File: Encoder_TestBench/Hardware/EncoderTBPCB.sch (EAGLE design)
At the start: 18 parts, among them IC1 7805DT, U1 ATMEGA328P-PU

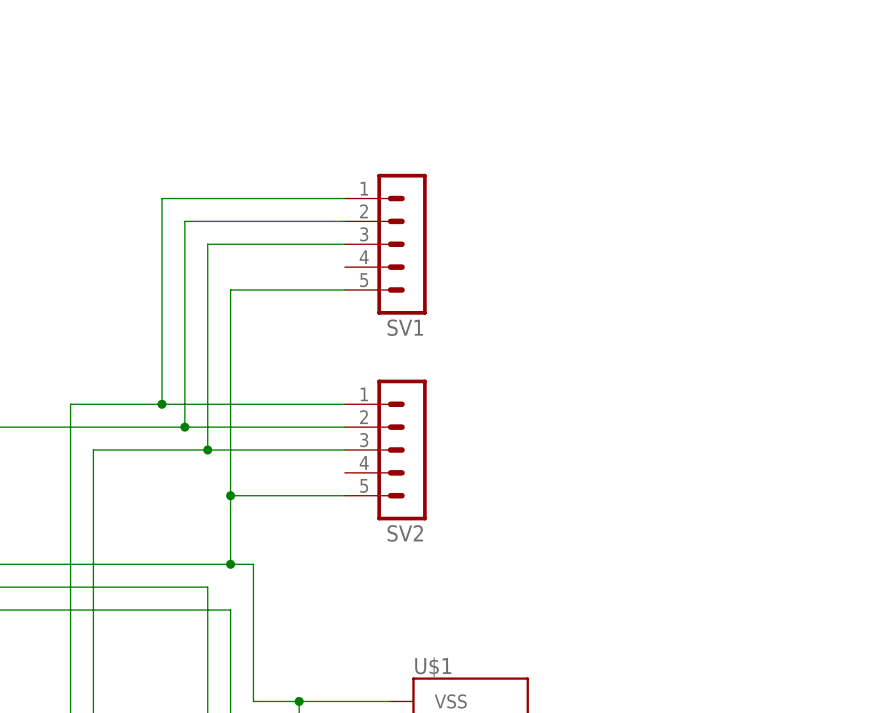
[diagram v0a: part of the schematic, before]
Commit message: Board Revised
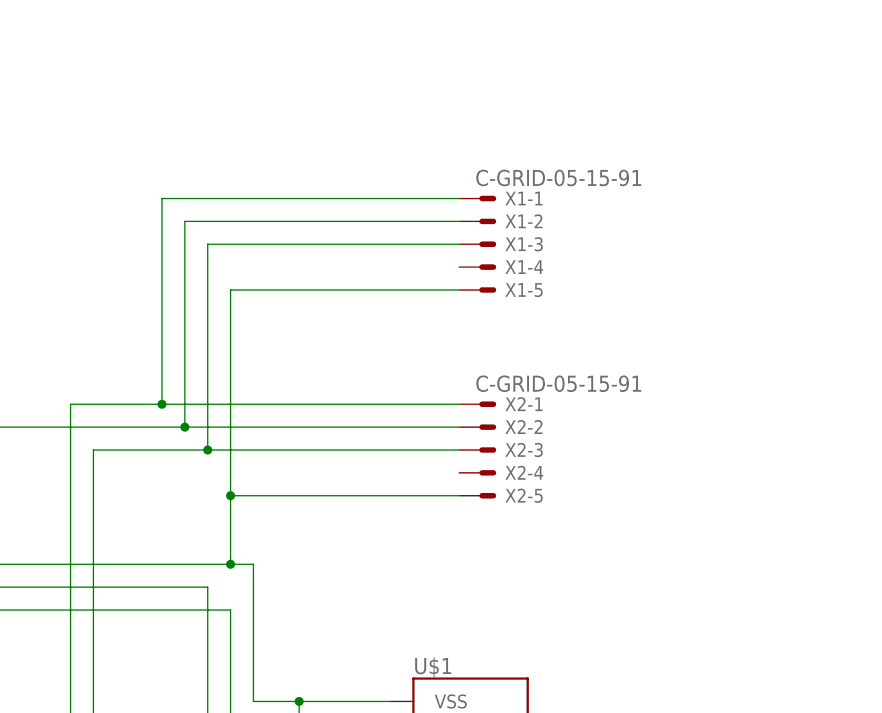
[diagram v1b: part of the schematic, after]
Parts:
- removed SV1, SV2: (no value), con-lstb:MA05-1
- added X1, X2: C-GRID-05-15-91, con-molex:C-GRID-05-15-91
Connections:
- net N$13: now also X1-1.S, X2-1.S; no longer SV1.1, SV2.1
- net N$14: now also X1-3.S, X2-3.S; no longer SV1.3, SV2.3
- net VDD: now also X1-2.S, X2-2.S; no longer SV1.2, SV2.2
- net VSS: now also X1-5.S, X2-5.S; no longer SV1.5, SV2.5
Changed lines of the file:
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@@
 <part name="R3" library="resistor" deviceset="R-US_" device="R0603" value="1MΩ"/>
 <part name="R4" library="resistor" deviceset="R-US_" device="R0603" value="850Ω"/>
-<part name="SV1" library="con-lstb" deviceset="MA05-1" device=""/>
-<part name="SV2" library="con-lstb" deviceset="MA05-1" device=""/>
 <part name="U$1" library="HD44780LCD" deviceset="LCD-HD44780" device="16X2-4-HOLES" technology="4-HOLES"/>
 <part name="R2" library="resistor" deviceset="R-US_" device="R0603" value="200Ω"/>
+<part name="X1" library="con-molex" deviceset="C-GRID-05" device="-15-91"/>
+<part name="X2" library="con-molex" deviceset="C-GRID-05" device="-15-91"/>
 </parts>
 <sheets>
@@
 <instance part="R3" gate="G$1" x="-5.08" y="43.18" rot="R90"/>
 <instance part="R4" gate="G$1" x="78.74" y="22.86" rot="R90"/>
-<instance part="SV1" gate="G$1" x="101.6" y="124.46" rot="R180"/>
-<instance part="SV2" gate="G$1" x="101.6" y="101.6" rot="R180"/>
 <instance part="U$1" gate="G$1" x="109.22" y="53.34"/>
 <instance part="R2" gate="G$1" x="66.04" y="15.24" rot="R180"/>
+<instance part="X1" gate="-1" x="109.22" y="129.54"/>
+<instance part="X1" gate="-2" x="109.22" y="127"/>
+<instance part="X1" gate="-3" x="109.22" y="124.46"/>
+<instance part="X1" gate="-4" x="109.22" y="121.92"/>
+<instance part="X1" gate="-5" x="109.22" y="119.38"/>
+<instance part="X2" gate="-1" x="109.22" y="106.68"/>
+<instance part="X2" gate="-2" x="109.22" y="104.14"/>
+<instance part="X2" gate="-3" x="109.22" y="101.6"/>
+<instance part="X2" gate="-4" x="109.22" y="99.06"/>
+<instance part="X2" gate="-5" x="109.22" y="96.52"/>
 </instances>
 <busses>
@@
 <junction x="81.28" y="88.9"/>
 <wire x1="81.28" y1="96.52" x2="81.28" y2="119.38" width="0.1524" layer="91"/>
-<wire x1="81.28" y1="96.52" x2="93.98" y2="96.52" width="0.1524" layer="91"/>
 <junction x="81.28" y="96.52"/>
 <wire x1="96.52" y1="5.08" x2="96.52" y2="35.56" width="0.1524" layer="91"/>
 <wire x1="96.52" y1="35.56" x2="99.06" y2="35.56" width="0.1524" layer="91"/>
-<pinref part="SV2" gate="G$1" pin="5"/>
 <pinref part="U1" gate="A" pin="GND_2"/>
 <pinref part="U1" gate="A" pin="GND"/>
@@
 <pinref part="U$1" gate="G$1" pin="R/W"/>
 <pinref part="U$1" gate="G$1" pin="VSS"/>
-<pinref part="SV1" gate="G$1" pin="5"/>
-<wire x1="81.28" y1="119.38" x2="93.98" y2="119.38" width="0.1524" layer="91"/>
 <pinref part="R2" gate="G$1" pin="2"/>
 <wire x1="60.96" y1="15.24" x2="58.42" y2="15.24" width="0.1524" layer="91"/>
 <junction x="58.42" y="15.24"/>
+<pinref part="X1" gate="-5" pin="S"/>
+<wire x1="81.28" y1="119.38" x2="106.68" y2="119.38" width="0.1524" layer="91"/>
+<pinref part="X2" gate="-5" pin="S"/>
+<wire x1="81.28" y1="96.52" x2="106.68" y2="96.52" width="0.1524" layer="91"/>
 </segment>
 <segment>
@@
 <wire x1="17.78" y1="104.14" x2="76.2" y2="104.14" width="0.1524" layer="91"/>
 <pinref part="JP1" gate="A" pin="2"/>
-<wire x1="76.2" y1="104.14" x2="93.98" y2="104.14" width="0.1524" layer="91"/>
+<wire x1="76.2" y1="104.14" x2="106.68" y2="104.14" width="0.1524" layer="91"/>
 <wire x1="2.54" y1="22.86" x2="7.62" y2="22.86" width="0.1524" layer="91"/>
 <wire x1="7.62" y1="22.86" x2="7.62" y2="27.94" width="0.1524" layer="91"/>
@@
 <wire x1="76.2" y1="104.14" x2="76.2" y2="127" width="0.1524" layer="91"/>
 <junction x="76.2" y="104.14"/>
-<wire x1="76.2" y1="127" x2="93.98" y2="127" width="0.1524" layer="91"/>
+<wire x1="76.2" y1="127" x2="106.68" y2="127" width="0.1524" layer="91"/>
 <pinref part="P+2" gate="1" pin="+5V"/>
-<pinref part="SV1" gate="G$1" pin="2"/>
-<pinref part="SV2" gate="G$1" pin="2"/>
 <wire x1="17.78" y1="73.66" x2="19.05" y2="73.66" width="0.1524" layer="91"/>
 <pinref part="U1" gate="A" pin="VCC"/>
 <pinref part="U1" gate="A" pin="AVCC"/>
+<pinref part="X1" gate="-2" pin="S"/>
+<pinref part="X2" gate="-2" pin="S"/>
 </segment>
 </net>
@@
 <segment>
 <wire x1="63.5" y1="106.68" x2="73.66" y2="106.68" width="0.1524" layer="91"/>
-<wire x1="73.66" y1="106.68" x2="93.98" y2="106.68" width="0.1524" layer="91"/>
+<wire x1="73.66" y1="106.68" x2="106.68" y2="106.68" width="0.1524" layer="91"/>
 <wire x1="73.66" y1="106.68" x2="73.66" y2="129.54" width="0.1524" layer="91"/>
 <junction x="73.66" y="106.68"/>
-<wire x1="73.66" y1="129.54" x2="93.98" y2="129.54" width="0.1524" layer="91"/>
-<pinref part="SV1" gate="G$1" pin="1"/>
-<pinref part="SV2" gate="G$1" pin="1"/>
+<wire x1="73.66" y1="129.54" x2="106.68" y2="129.54" width="0.1524" layer="91"/>
 <wire x1="63.5" y1="106.68" x2="63.5" y2="71.12" width="0.1524" layer="91"/>
 <wire x1="63.5" y1="71.12" x2="54.61" y2="71.12" width="0.1524" layer="91"/>
 <pinref part="U1" gate="A" pin="PD1"/>
+<pinref part="X1" gate="-1" pin="S"/>
+<pinref part="X2" gate="-1" pin="S"/>
 </segment>
 </net>
@@
 <segment>
 <wire x1="66.04" y1="101.6" x2="78.74" y2="101.6" width="0.1524" layer="91"/>
-<wire x1="78.74" y1="101.6" x2="93.98" y2="101.6" width="0.1524" layer="91"/>
+<wire x1="78.74" y1="101.6" x2="106.68" y2="101.6" width="0.1524" layer="91"/>
 <wire x1="78.74" y1="101.6" x2="78.74" y2="124.46" width="0.1524" layer="91"/>
 <junction x="78.74" y="101.6"/>
-<wire x1="78.74" y1="124.46" x2="93.98" y2="124.46" width="0.1524" layer="91"/>
-<pinref part="SV1" gate="G$1" pin="3"/>
-<pinref part="SV2" gate="G$1" pin="3"/>
+<wire x1="78.74" y1="124.46" x2="106.68" y2="124.46" width="0.1524" layer="91"/>
 <wire x1="66.04" y1="101.6" x2="66.04" y2="68.58" width="0.1524" layer="91"/>
 <wire x1="66.04" y1="68.58" x2="54.61" y2="68.58" width="0.1524" layer="91"/>
 <pinref part="U1" gate="A" pin="PD2"/>
-</segment>
-</net>
+<pinref part="X1" gate="-3" pin="S"/>
+<pinref part="X2" gate="-3" pin="S"/>
+</segment>
+</net>

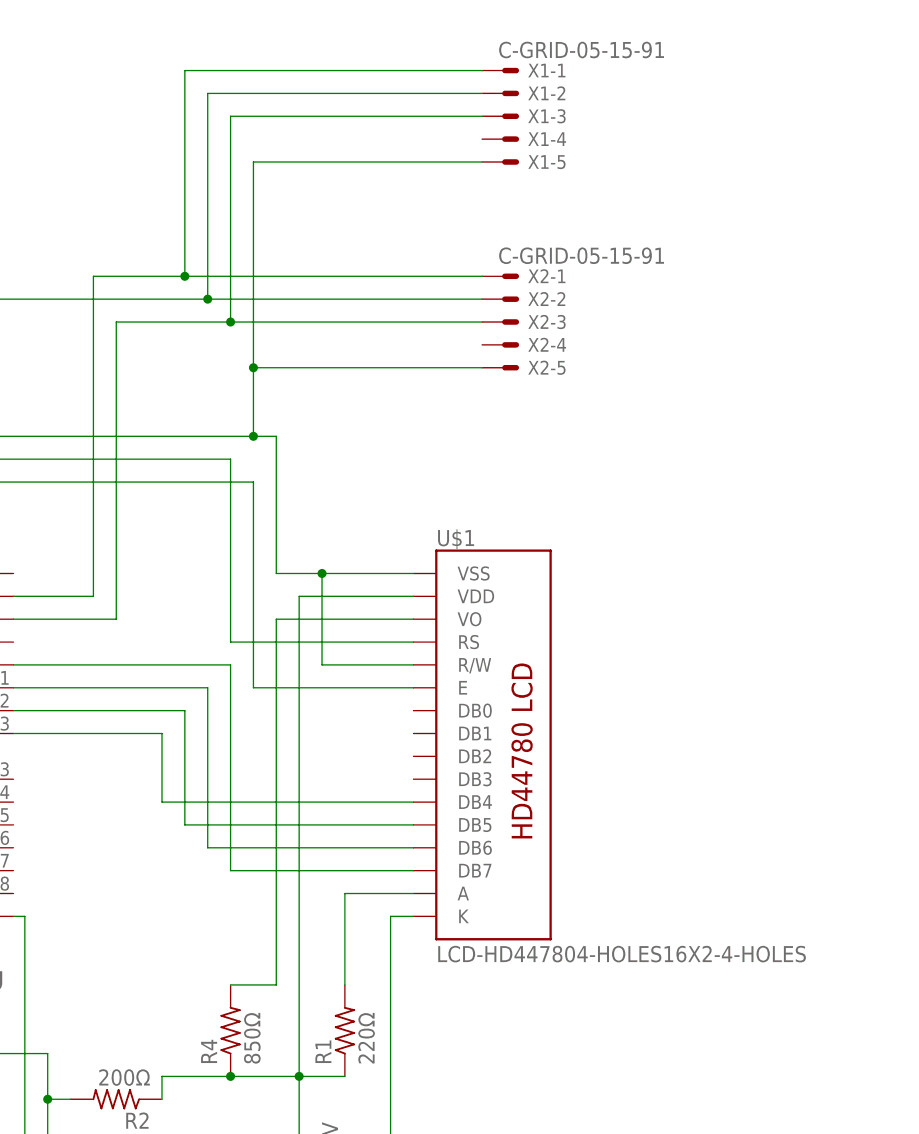
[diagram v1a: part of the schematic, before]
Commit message: Port Updated
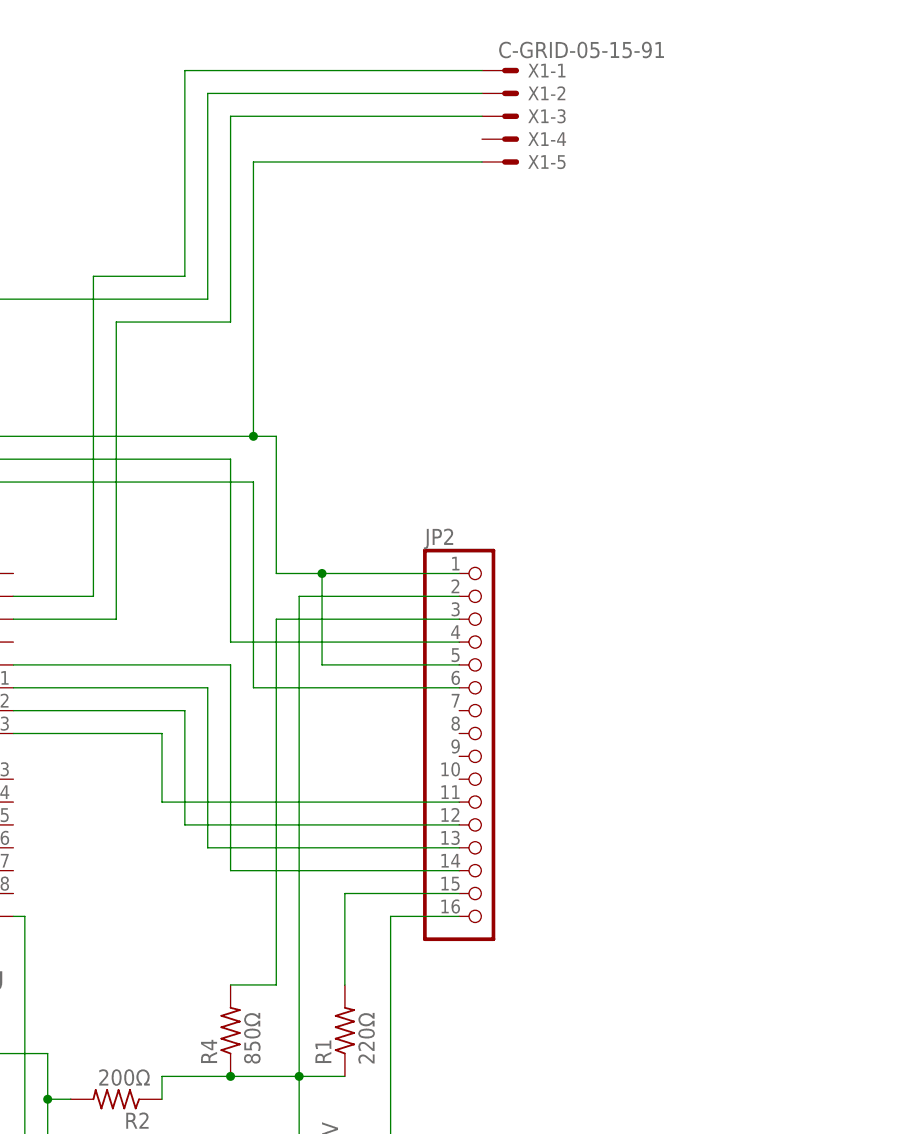
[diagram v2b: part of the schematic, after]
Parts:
- removed U$1: LCD-HD447804-HOLES16X2-4-HOLES, HD44780LCD:LCD-HD447804-HOLES16X2-4-HOLES
- removed X2: C-GRID-05-15-91, con-molex:C-GRID-05-15-91
- added JP2: (no value), pinhead:PINHD-1X16
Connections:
- net N$1: now also JP2.6; no longer U$1.E
- net N$13: no longer X2-1.S
- net N$14: no longer X2-3.S
- net N$2: now also JP2.15; no longer U$1.A
- net N$4: now also JP2.14; no longer U$1.DB7
- net N$5: now also JP2.13; no longer U$1.DB6
- net N$6: now also JP2.12; no longer U$1.DB5
- net N$7: now also JP2.11; no longer U$1.DB4
- net N$9: now also JP2.4; no longer U$1.RS
- net VDD: now also JP2.2; no longer U$1.VDD, X2-2.S
- net VO: now also JP2.3; no longer U$1.VO
- net VSS: now also JP2.1, JP2.16, JP2.5; no longer U$1.K, U$1.R/W, U$1.VSS, X2-5.S
